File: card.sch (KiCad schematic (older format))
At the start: 0 parts

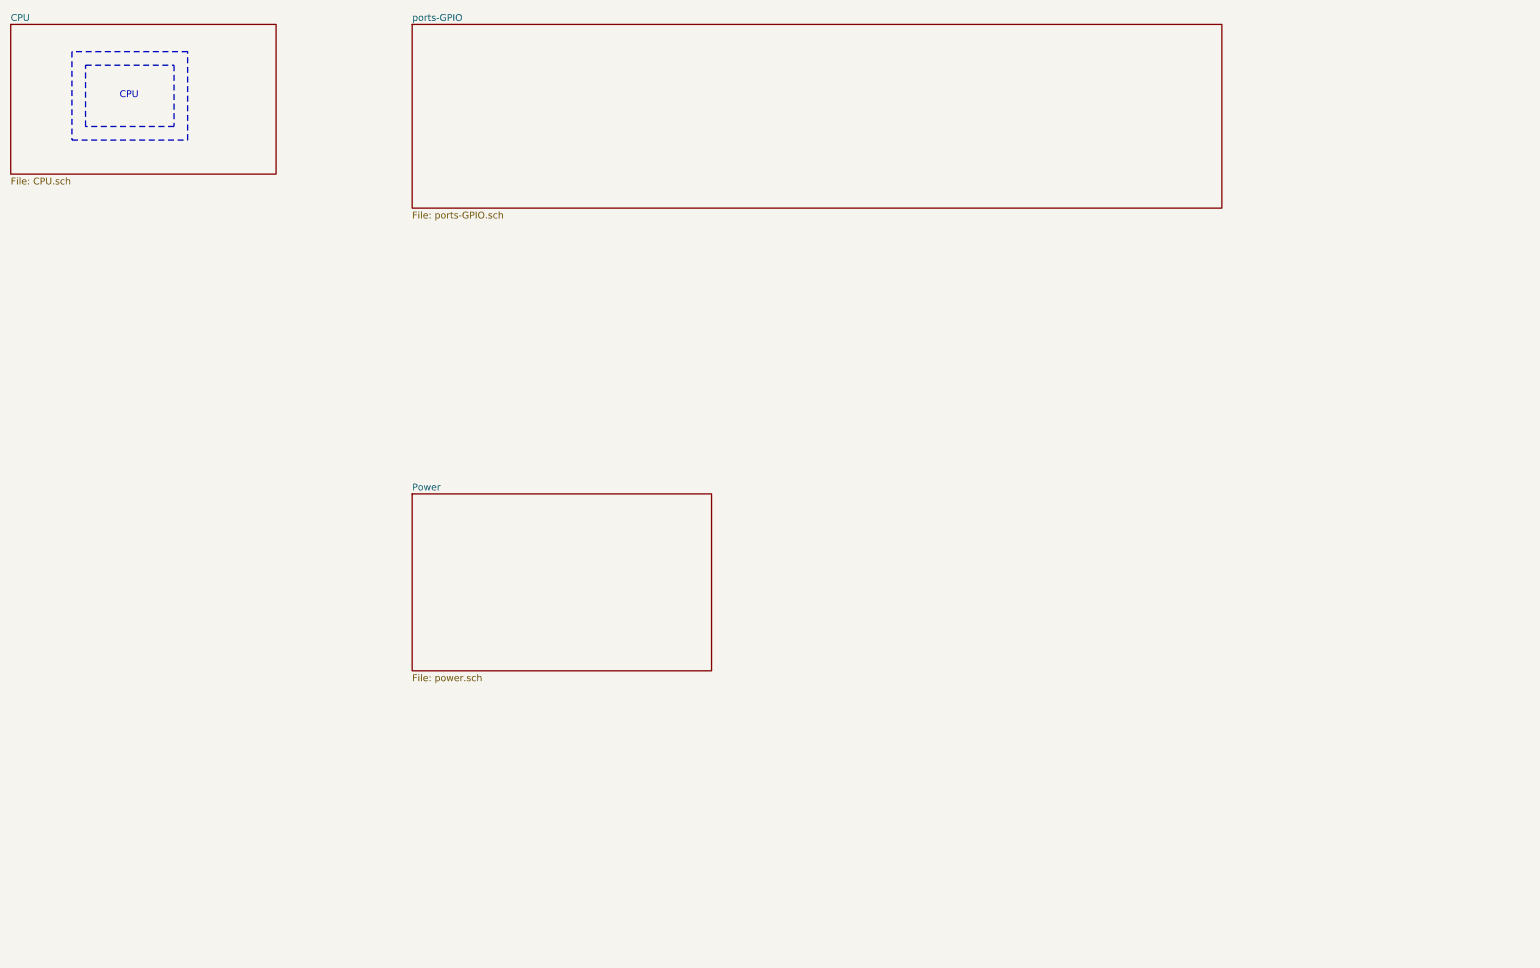
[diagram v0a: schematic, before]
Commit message: added todo list before i feel aleeped on my keybard*
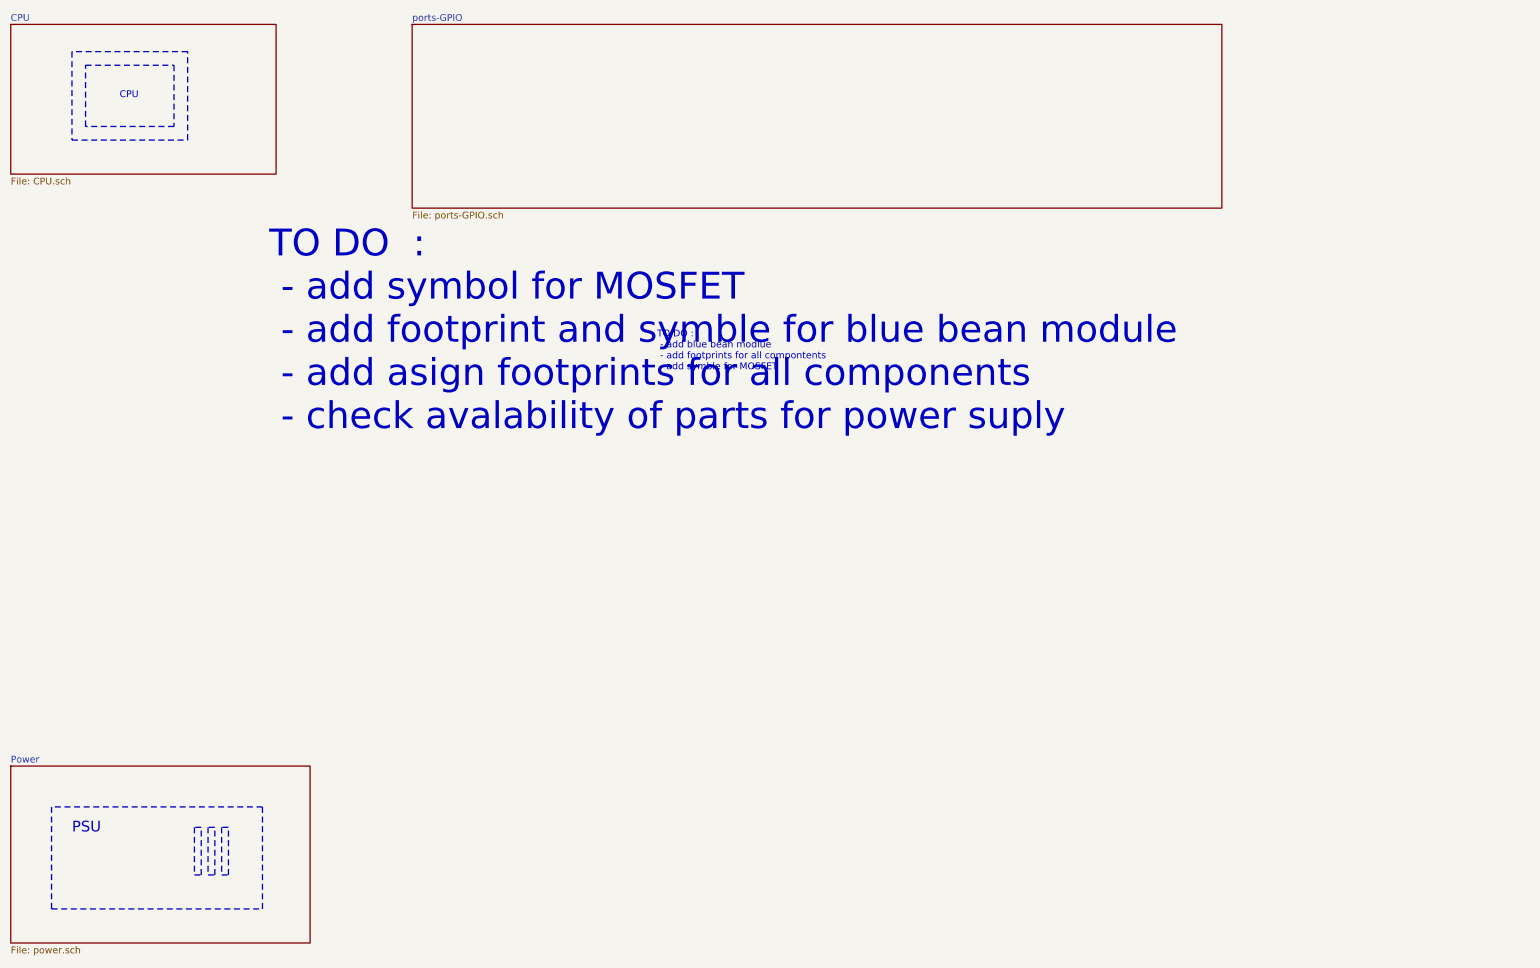
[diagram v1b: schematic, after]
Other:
- note added: "PSU"
- note added: "TO DO :\n - add blue bean modlue \n - add footprints for all compontents\n - add symble for MOSFET"
- note added: "TO DO :\n - add symbol for MOSFET\n - add footprint and symble for blue bean module\n - add asign footprints for all components\n - check avalability of parts for power suply"
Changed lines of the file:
@@
 $EndDescr
 $Sheet
-S 3800 4250 2200 1300
+S 850  6250 2200 1300
 U 5F46881F
 F0 "Power" 50
@@
 F1 "ports-GPIO.sch" 50
 $EndSheet
+Text Notes 5600 3350 0    0    ~ 0
+TO DO :\n - add blue bean modlue \n - add footprints for all compontents\n - add symble for MOSFET
+Text Notes 2750 3800 0    197  ~ 0
+TO DO  :\n - add symbol for MOSFET\n - add footprint and symble for blue bean module\n - add asign footprints for all components\n - check avalability of parts for power suply
+Wire Notes Line
+	1150 6550 1150 7300
+Wire Notes Line
+	1150 7300 2700 7300
+Wire Notes Line
+	2700 7300 2700 6550
+Wire Notes Line
+	2700 6550 1150 6550
+Wire Notes Line
+	2200 6700 2200 7050
+Wire Notes Line
+	2200 7050 2250 7050
+Wire Notes Line
+	2250 7050 2250 6700
+Wire Notes Line
+	2250 6700 2200 6700
+Wire Notes Line
+	2300 6700 2300 7050
+Wire Notes Line
+	2300 7050 2350 7050
+Wire Notes Line
+	2350 7050 2350 6700
+Wire Notes Line
+	2350 6700 2300 6700
+Wire Notes Line
+	2400 6700 2400 7050
+Wire Notes Line
+	2400 7050 2450 7050
+Wire Notes Line
+	2450 7050 2450 6700
+Wire Notes Line
+	2450 6700 2400 6700
+Text Notes 1300 6750 0    79   ~ 0
+PSU
 $EndSCHEMATC
